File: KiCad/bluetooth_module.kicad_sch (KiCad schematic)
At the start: 10 parts, among them U10 SN74LV1T34DCK, U11 RN4871, U12 LM810, U13 SN74LV1T34DCK, U9 SN74LV1T34DCK

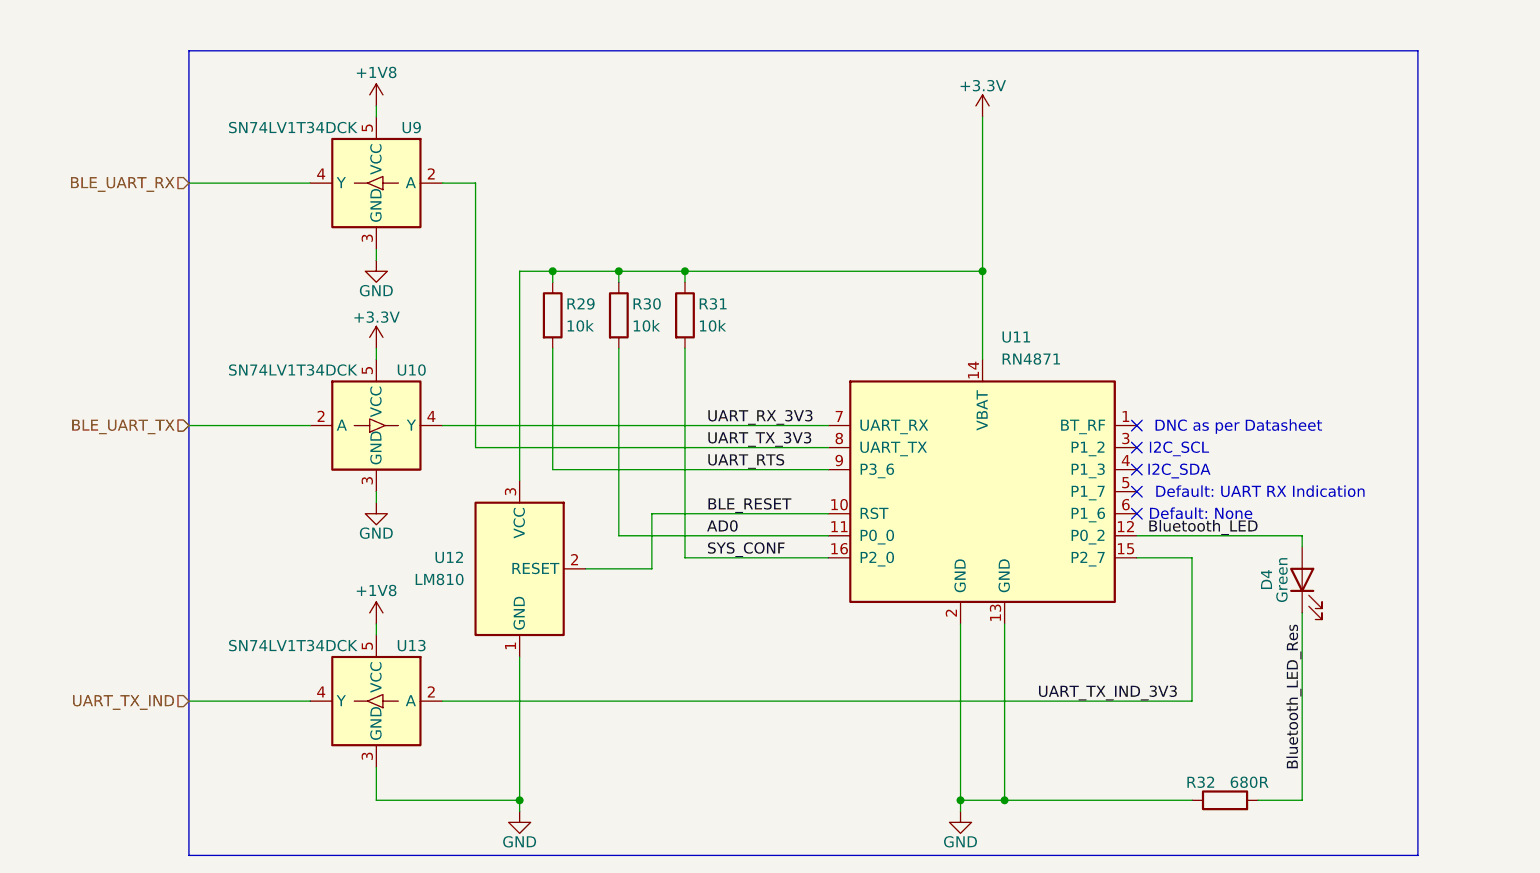
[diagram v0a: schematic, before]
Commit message: Added some TODOs, fixed some TODOs
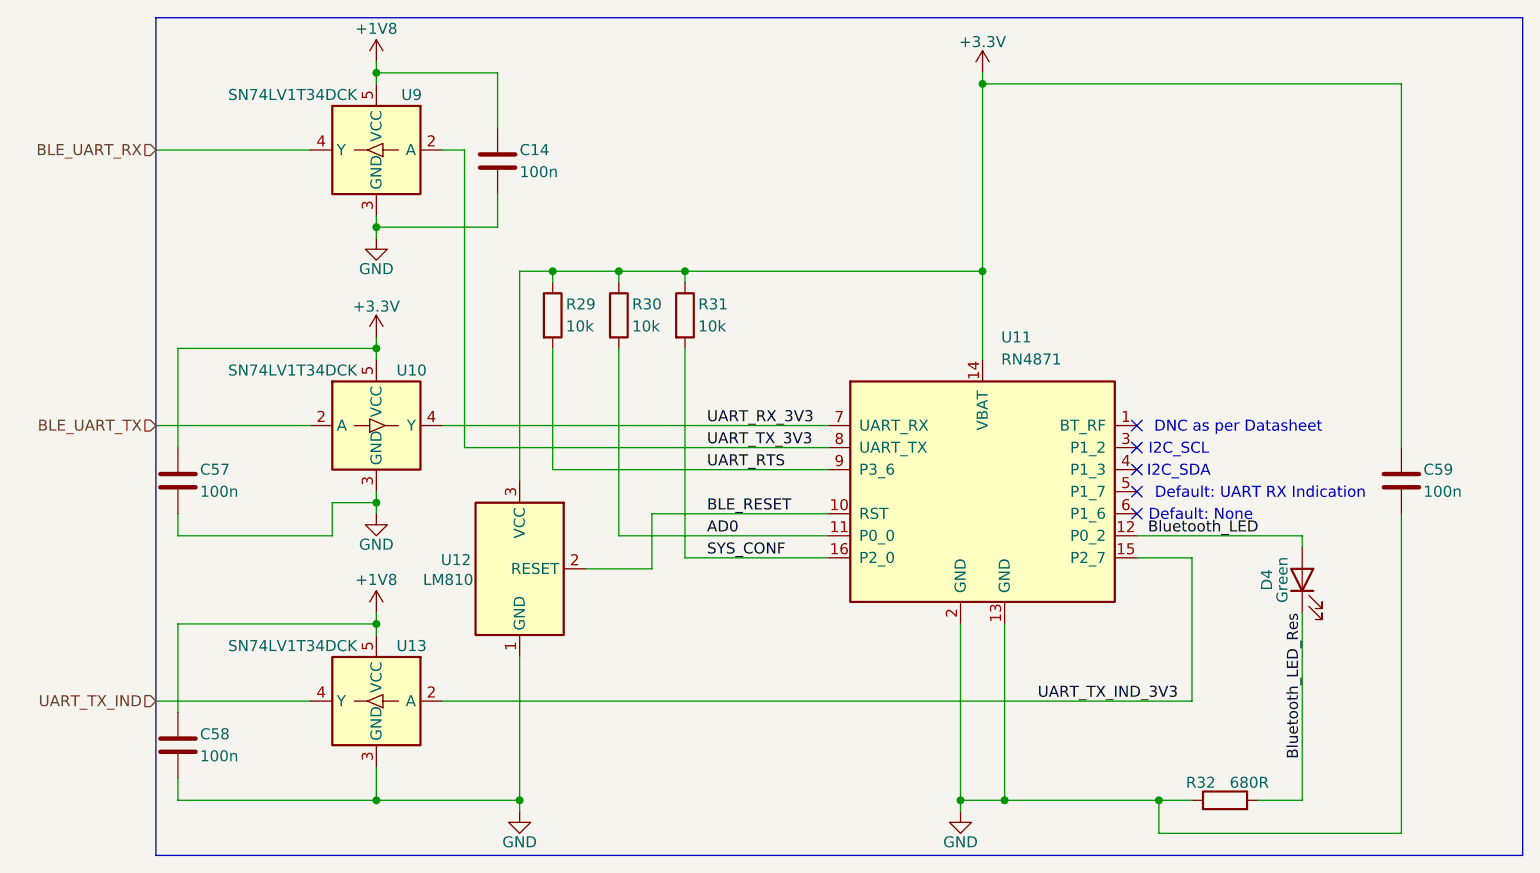
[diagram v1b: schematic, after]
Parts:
- added C14, C57, C58, C59: 100n, Capacitor_SMD:C_0402_1005Metric, symbol Device:C
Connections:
- net +1V8: now also C14.1, C58.1
- net +3.3V: now also C57.1, C59.1
- net GND: now also C14.2, C57.2, C58.2, C59.2
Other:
- moved on the sheet: U9
